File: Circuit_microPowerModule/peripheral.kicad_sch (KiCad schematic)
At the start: 34 parts, among them J501 HDR-2.54 Male 1x5, J503 HDR-2.54 Female 1x5, J6 MikroBus

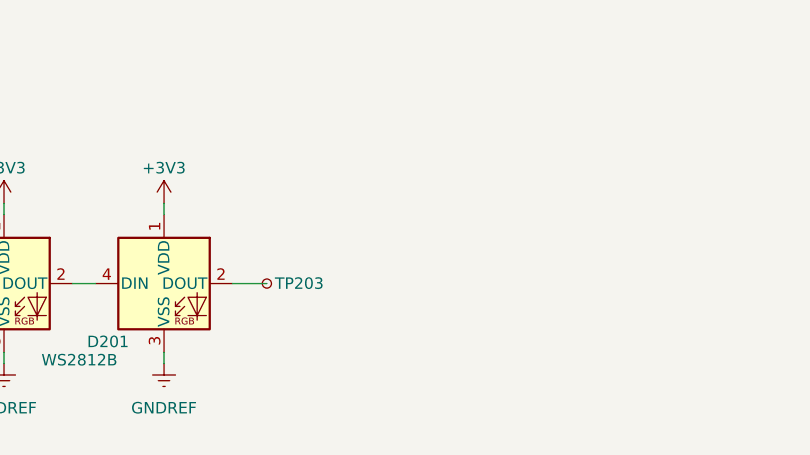
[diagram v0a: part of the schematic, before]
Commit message: set board edge cut
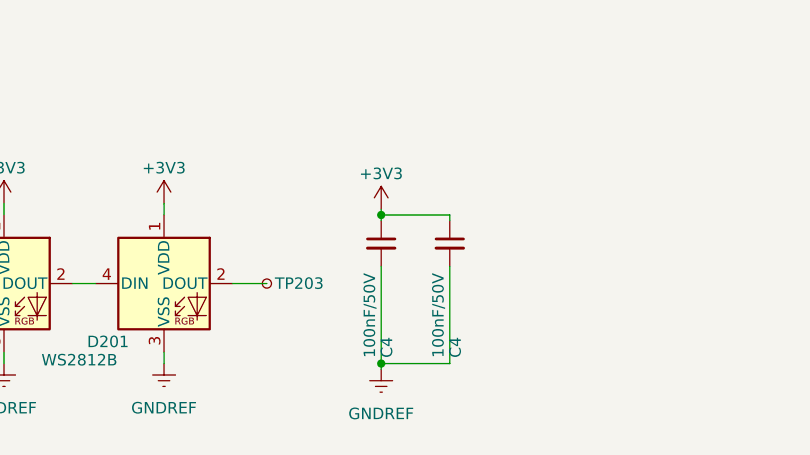
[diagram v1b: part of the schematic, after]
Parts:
- added C4 (x2): 100nF/50V, Capacitor_SMD:C_0603_1608Metric, symbol Device:C_Small
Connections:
- net +3V3: now also C4.1, C4.1
- net GNDREF: now also C4.2, C4.2
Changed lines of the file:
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@@
   (junction (at 69.85 53.34) (diameter 0) (color 0 0 0 0)
   )
+  (junction (at 90.17 177.8) (diameter 0) (color 0 0 0 0)
+  )
   (junction (at 69.85 45.72) (diameter 0) (color 0 0 0 0)
   )
@@
   )
   (junction (at 165.1 140.97) (diameter 0) (color 0 0 0 0)
+  )
+  (junction (at 90.17 161.29) (diameter 0) (color 0 0 0 0)
   )
   (junction (at 69.85 113.03) (diameter 0) (color 0 0 0 0)
@@
     (stroke (width 0) (type default))
   )
+  (wire (pts (xy 97.79 177.8) (xy 90.17 177.8))
+    (stroke (width 0) (type default))
+  )
   (wire (pts (xy 190.5 129.54) (xy 209.55 129.54))
     (stroke (width 0) (type default))
@@
     (stroke (width 0) (type default))
   )
+  (wire (pts (xy 97.79 161.29) (xy 90.17 161.29))
+    (stroke (width 0) (type default))
+  )
   (wire (pts (xy 219.71 54.61) (xy 226.06 54.61))
     (stroke (width 0) (type default))
@@
     (stroke (width 0) (type default))
   )
+  (wire (pts (xy 90.17 167.005) (xy 90.17 177.8))
+    (stroke (width 0) (type default))
+  )
   (wire (pts (xy 146.05 129.54) (xy 167.64 129.54))
     (stroke (width 0) (type default))
@@
     (stroke (width 0) (type default))
   )
+  (wire (pts (xy 90.17 161.29) (xy 90.17 161.925))
+    (stroke (width 0) (type default))
+  )
   (wire (pts (xy 111.76 52.07) (xy 123.825 52.07))
     (stroke (width 0) (type default))
@@
     (stroke (width 0) (type default))
   )
+  (wire (pts (xy 97.79 161.925) (xy 97.79 161.29))
+    (stroke (width 0) (type default))
+  )
   (wire (pts (xy 44.45 49.53) (xy 44.45 50.8))
     (stroke (width 0) (type default))
   )
+  (wire (pts (xy 90.17 177.8) (xy 90.17 178.435))
+    (stroke (width 0) (type default))
+  )
   (wire (pts (xy 208.28 57.15) (xy 210.82 57.15))
     (stroke (width 0) (type default))
@@
     (stroke (width 0) (type default))
   )
+  (wire (pts (xy 97.79 167.005) (xy 97.79 177.8))
+    (stroke (width 0) (type default))
+  )
   (wire (pts (xy 49.53 115.57) (xy 49.53 127))
     (stroke (width 0) (type default))
@@
   )
   (wire (pts (xy 44.45 49.53) (xy 36.83 49.53))
+    (stroke (width 0) (type default))
+  )
+  (wire (pts (xy 90.17 160.655) (xy 90.17 161.29))
     (stroke (width 0) (type default))
   )
@@
     )
   )
+  (symbol (lib_id "power:GNDREF") (at 90.17 178.435 0) (mirror y) (unit 1)
+    (in_bom yes) (on_board yes) (dnp no) (fields_autoplaced)
+    (property "Reference" "#PWR0220" (at 90.17 184.785 0)
+      (effects (font (size 1.27 1.27)) hide)
+    )
+    (property "Value" "GNDREF" (at 90.17 183.388 0)
+      (effects (font (size 1.27 1.27)))
+    )
+    (property "Footprint" "" (at 90.17 178.435 0)
+      (effects (font (size 1.27 1.27)) hide)
+    )
+    (property "Datasheet" "" (at 90.17 178.435 0)
+      (effects (font (size 1.27 1.27)) hide)
+    )
+    (pin "1")
+    (instances
+      (project "micro-PowerModule"
+        (path "/38b19d1a-a8d3-49c0-a6a2-bee4e845832f/7187d72d-86a6-4df3-a706-10f93237b261"
+          (reference "#PWR0220") (unit 1)
+        )
+        (path "/38b19d1a-a8d3-49c0-a6a2-bee4e845832f/ff7f9ef2-679c-4e45-a086-9ba6ae131839"
+          (reference "#PWR0521") (unit 1)
+        )
+      )
+    )
+  )
   (symbol (lib_id "power:VBUS") (at 116.205 38.1 0) (unit 1)
     (in_bom yes) (on_board yes) (dnp no) (fields_autoplaced)
@@
         (path "/38b19d1a-a8d3-49c0-a6a2-bee4e845832f/ff7f9ef2-679c-4e45-a086-9ba6ae131839"
           (reference "#FLG0501") (unit 1)
+        )
+      )
+    )
+  )
+  (symbol (lib_id "power:+3V3") (at 90.17 160.655 0) (mirror y) (unit 1)
+    (in_bom yes) (on_board yes) (dnp no) (fields_autoplaced)
+    (property "Reference" "#PWR0219" (at 90.17 164.465 0)
+      (effects (font (size 1.27 1.27)) hide)
+    )
+    (property "Value" "+3V3" (at 90.17 156.718 0)
+      (effects (font (size 1.27 1.27)))
+    )
+    (property "Footprint" "" (at 90.17 160.655 0)
+      (effects (font (size 1.27 1.27)) hide)
+    )
+    (property "Datasheet" "" (at 90.17 160.655 0)
+      (effects (font (size 1.27 1.27)) hide)
+    )
+    (pin "1")
+    (instances
+      (project "micro-PowerModule"
+        (path "/38b19d1a-a8d3-49c0-a6a2-bee4e845832f/7187d72d-86a6-4df3-a706-10f93237b261"
+          (reference "#PWR0219") (unit 1)
+        )
+        (path "/38b19d1a-a8d3-49c0-a6a2-bee4e845832f/ff7f9ef2-679c-4e45-a086-9ba6ae131839"
+          (reference "#PWR0520") (unit 1)
         )
       )
@@
         (path "/38b19d1a-a8d3-49c0-a6a2-bee4e845832f/ff7f9ef2-679c-4e45-a086-9ba6ae131839"
           (reference "JP505") (unit 1)
+        )
+      )
+    )
+  )
+  (symbol (lib_id "Device:C_Small") (at 90.17 164.465 0) (unit 1)
+    (in_bom yes) (on_board yes) (dnp no)
+    (property "Reference" "C4" (at 90.805 177.165 90)
+      (effects (font (size 1.27 1.27)) (justify left))
+    )
+    (property "Value" "100nF/50V" (at 88.9 177.165 90)
+      (effects (font (size 1.27 1.27)) (justify left))
+    )
+    (property "Footprint" "Capacitor_SMD:C_0603_1608Metric" (at 90.17 164.465 0)
+      (effects (font (size 1.27 1.27)) hide)
+    )
+    (property "Datasheet" "~" (at 90.17 164.465 0)
+      (effects (font (size 1.27 1.27)) hide)
+    )
+    (pin "1")
+    (pin "2")
+    (instances
+      (project "micro-PowerModule"
+        (path "/38b19d1a-a8d3-49c0-a6a2-bee4e845832f/4d2335ad-4917-40e3-b9fc-5e8d69783b2a"
+          (reference "C4") (unit 1)
+        )
+        (path "/38b19d1a-a8d3-49c0-a6a2-bee4e845832f"
+          (reference "C?") (unit 1)
+        )
+        (path "/38b19d1a-a8d3-49c0-a6a2-bee4e845832f/ff7f9ef2-679c-4e45-a086-9ba6ae131839"
+          (reference "C505") (unit 1)
         )
       )
@@
         )
       )
+    )
+  )
+  (symbol (lib_id "Device:C_Small") (at 97.79 164.465 0) (unit 1)
+    (in_bom yes) (on_board yes) (dnp no)
+    (property "Reference" "C4" (at 98.425 177.165 90)
+      (effects (font (size 1.27 1.27)) (justify left))
+    )
+    (property "Value" "100nF/50V" (at 96.52 177.165 90)
+      (effects (font (size 1.27 1.27)) (justify left))
+    )
+    (property "Footprint" "Capacitor_SMD:C_0603_1608Metric" (at 97.79 164.465 0)
+      (effects (font (size 1.27 1.27)) hide)
+    )
+    (property "Datasheet" "~" (at 97.79 164.465 0)
+      (effects (font (size 1.27 1.27)) hide)
+    )
+    (pin "1")
+    (pin "2")
+    (instances
+      (project "micro-PowerModule"
+        (path "/38b19d1a-a8d3-49c0-a6a2-bee4e845832f/4d2335ad-4917-40e3-b9fc-5e8d69783b2a"
+          (reference "C4") (unit 1)
+        )
+        (path "/38b19d1a-a8d3-49c0-a6a2-bee4e845832f"
+          (reference "C?") (unit 1)
+        )
+        (path "/38b19d1a-a8d3-49c0-a6a2-bee4e845832f/ff7f9ef2-679c-4e45-a086-9ba6ae131839"
+          (reference "C506") (unit 1)
+        )
+      )
